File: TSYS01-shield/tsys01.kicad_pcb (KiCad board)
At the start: 2 copper layers, 20 x 24 mm, 25 parts, among them P1 CONN_01X02, P2 CONN_01X04, U1 TSYS01, U2 SP6213

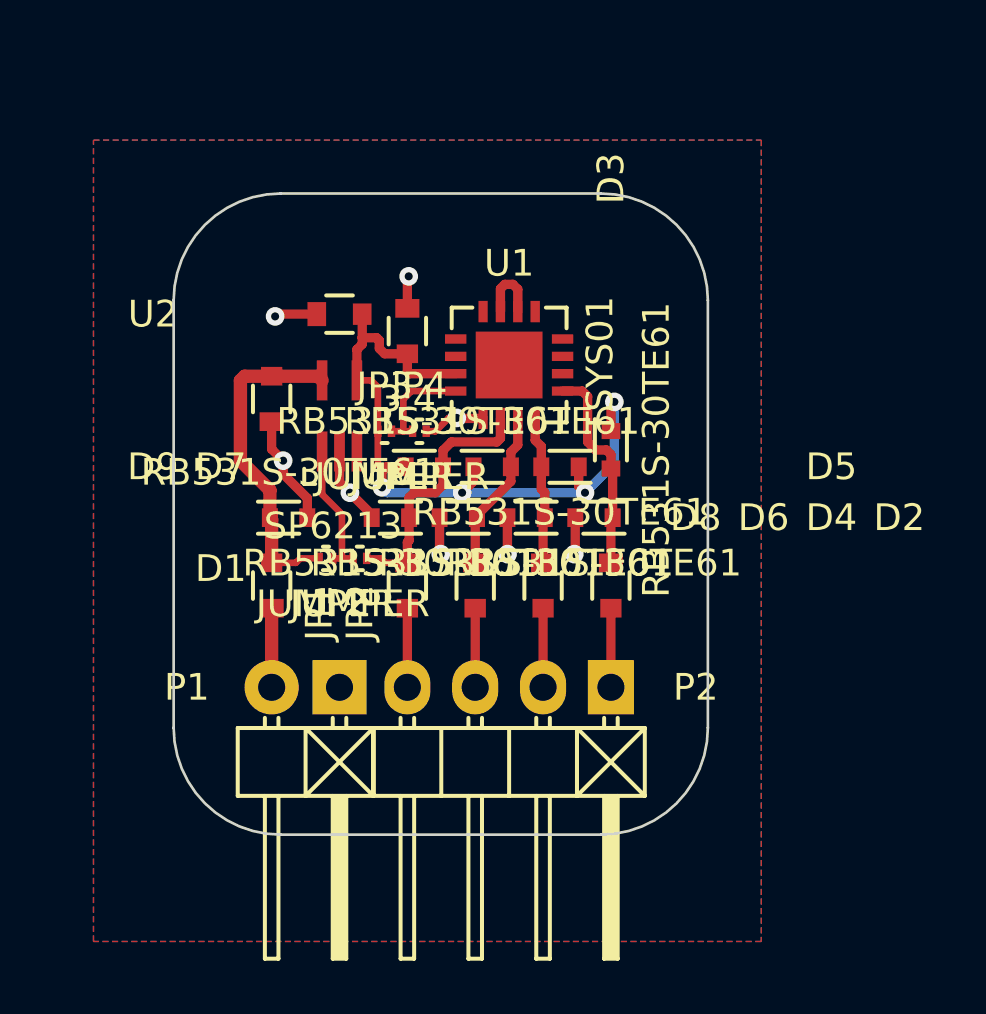
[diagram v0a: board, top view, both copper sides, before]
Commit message: First production version
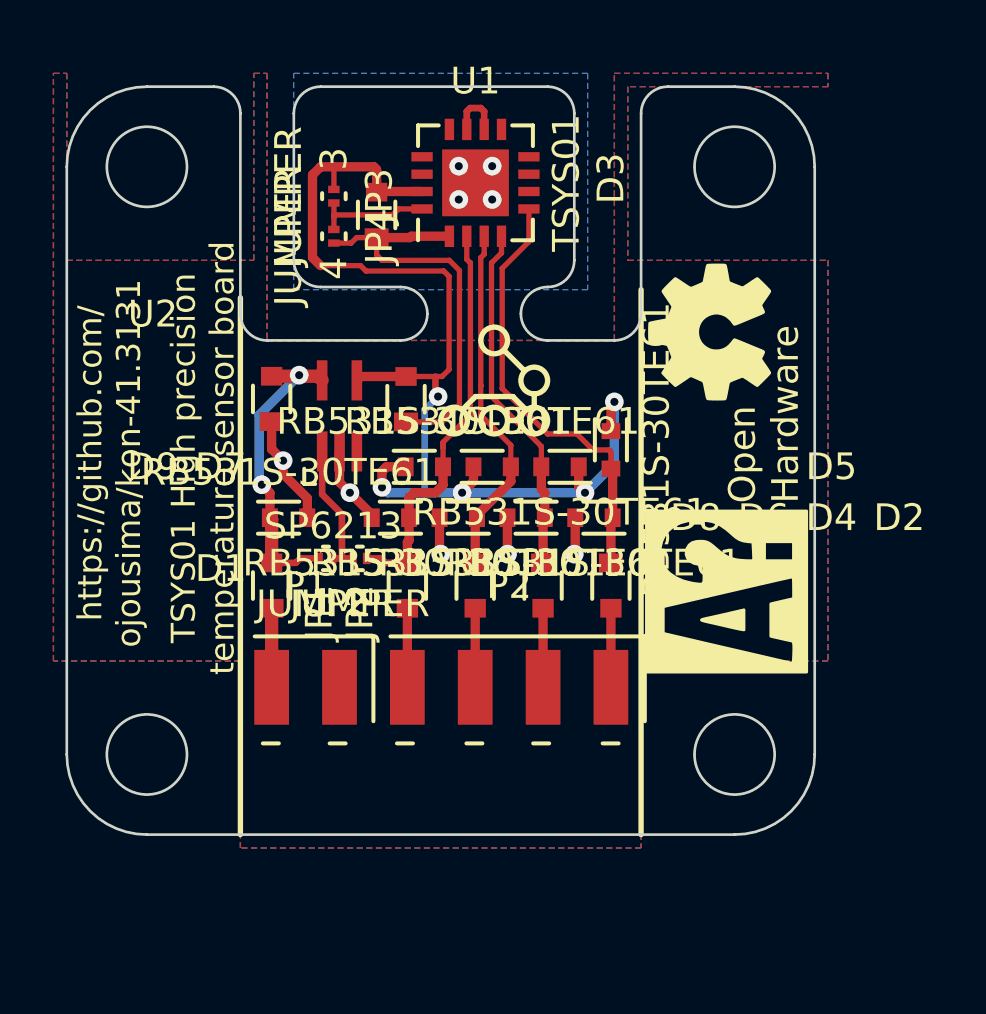
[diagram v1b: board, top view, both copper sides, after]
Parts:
- added G***: LOGO, LOGO, F.Cu at (43.1, 57.2)
- added G***: LOGO, LOGO, F.Cu at (43.7, 66.9)
- P1: footprint Pin_Headers:Pin_Header_Angled_1x02 -> pin_header_fork:Pin_Header_Angled_SMD_1x02
- P2: footprint Pin_Headers:Pin_Header_Angled_1x04 -> pin_header_fork:Pin_Header_Angled_SMD_1x04
- moved JP3 9.00 mm to (29.0, 52.1), turned to 270 degrees
- moved JP4 7.97 mm to (29.0, 53.6), turned to 270 degrees
- moved U1 6.94 mm to (34.3, 51.6)
- moved C3 4.50 mm to (30.6, 52.8), turned to 270 degrees
- moved C2 4.04 mm to (31.7, 59.7), turned to 270 degrees
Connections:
- U1 pad 17: (no net) -> /PAD
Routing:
- net +3V3: track 27.7 -> 42.9 mm, vias 4 -> 5
- net GNDA: track 16.4 -> 27.1 mm, vias 8 -> 5
- net Net-(D2-Pad2): track 8.02 -> 16.5 mm
- net Net-(D4-Pad2): track 5.58 -> 13.2 mm
- net Net-(D6-Pad2): track 6.07 -> 13.3 mm
- net /PAD: track 0.00 -> 5.97 mm, vias 0 -> 4
- net /EN: track 9.90 -> 15.4 mm
- net /Vin: track 12.3 -> 11.8 mm, vias 0 -> 2
- added copper zone on B.Cu, net /PAD
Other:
- board size 20 x 24 mm -> 28 x 28 mm
- net class Default: clearance 0.2 -> 0.19
- rule trace_clearance: 0.2 -> 0.19
- board text added: "5V"
- board text added: "CS"
- board text added: "GND"
- board text added: "I2C mode: R2 NO-POP, I2C Address: D8 Pull down OR D9 Pull up"
- board text added: "JMP1: always ON JMP2: ON when CS HIGH !JMP1 & !JMP2: undefined JMP1 & JMP2: short circuit"
- board text added: "JMP3: I2C mode JMP4: SPI mode !JMP3 & !JMP4: undefined JMP3 & JMP4: short circuit"
- board text added: "MISO"
- board text added: "MOSI/SDA"
- board text added: "Open Hardware"
- board text added: "SCLK/SCL"
- board text added: "SPI MODE: JMP1 only"
- board text added: "TSYS01 High precision temperature sensor board"
- board text added: "https://github.com/ ojousima/kon-41.3131"
